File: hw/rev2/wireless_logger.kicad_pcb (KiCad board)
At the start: 4 copper layers, 147 parts, among them J1 FCI 10118194, J2 CONN_2, J3 SSD1306_SER, J4 SWD_10PIN, J5 CONN_5, P1 CONN_6X2, Q1 2N7002P, Q2 2N7002P, U1 MT29FXX01A, U10 CC2541, U11 STM32F40X_BGA176, U2 MAG3110, U3 MMA8452Q, U4 LPS331AP, U5 L3GD20, U6 MCP111T-315, U7 BQ24095, U8 TPS62698, U9 CC1101, X1 FA-128 26.0000MF10Z-W3, X2 9HT10-32.768KBZF-T, X3 FA-128 32.0000MF20X-K3, X4 XRCGB25M000F0L00R0, X5 9HT10-32.768KBZF-T

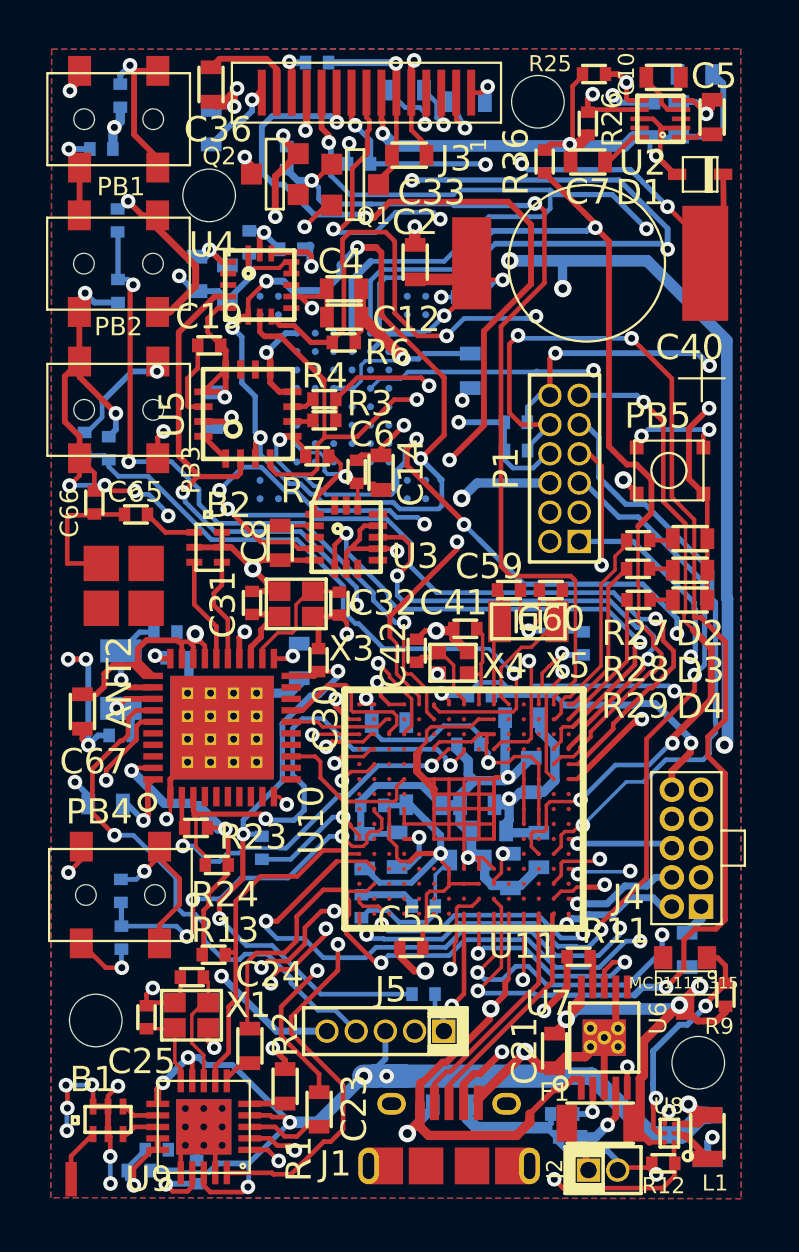
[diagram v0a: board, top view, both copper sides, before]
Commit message: Rev 2a submitted to OSH Park for manufacture
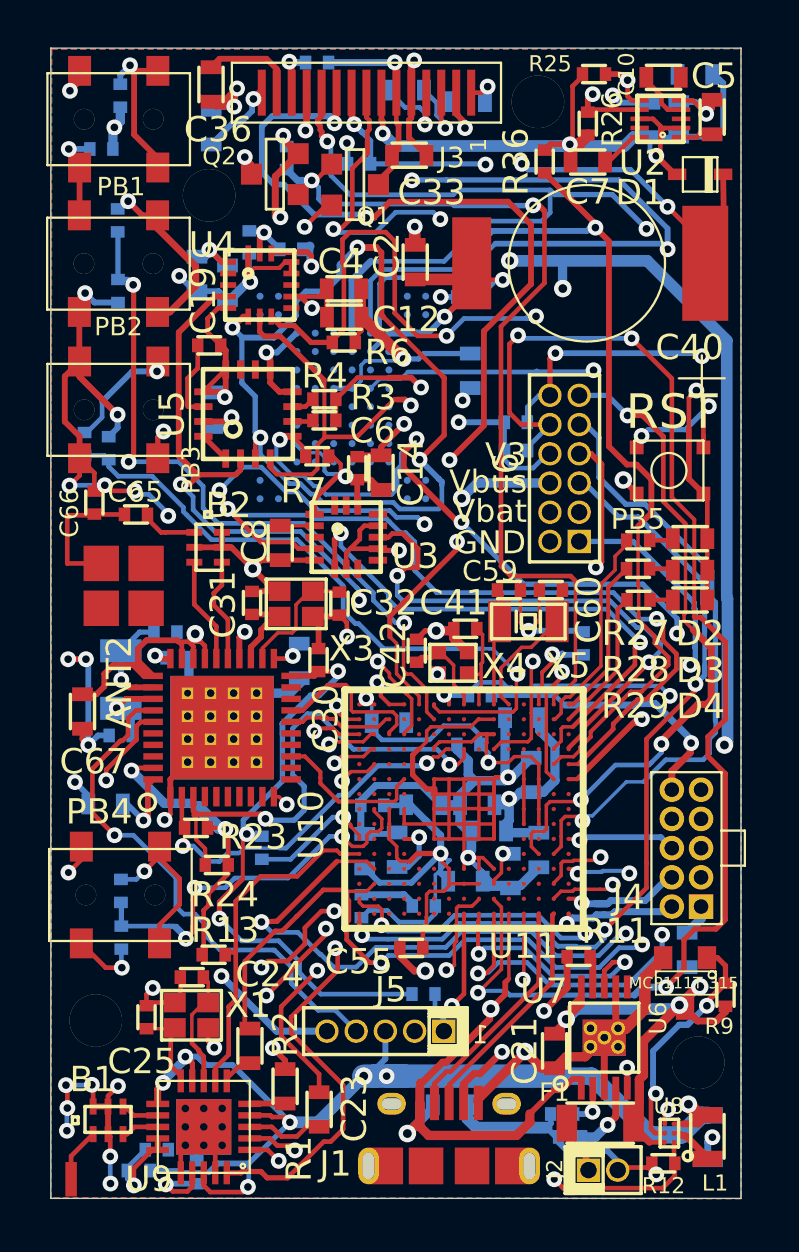
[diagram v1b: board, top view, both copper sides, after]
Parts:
- moved C50 0.92 mm to (188.0, 146.2)
- moved C6 0.16 mm to (183.3, 128.3)
- renumbered P1 to J6
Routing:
- net GND: track 269.3 -> 282.2 mm
- net N-00000167: track 28.6 -> 34.2 mm
- net /Sensors/GYR_SPI_MOSI: track 80.8 -> 85.1 mm, vias 7 -> 6
- net V3: track 328.2 -> 332.4 mm
- net /STM32F4/SPI2_NSS: track 51.5 -> 53.5 mm
- net /STM32F4/EXTI8: track 16.8 -> 18.6 mm
- net N-00000189: track 10.3 -> 12.1 mm
- net /STM32F4/OLED_nD/C: track 47.0 -> 48.6 mm
- net /Sensors/ACC_INT1: track 22.3 -> 23.8 mm
- net /Sensors/ACC_I2C_SCL: track 66.3 -> 67.7 mm
- net /Sensors/GYR_SPI_MISO: track 63.3 -> 62.1 mm
- net /Bluetooth/RF_RESET_N_LOCAL: track 25.8 -> 26.9 mm
- net /OLED/OLED_GND: track 19.3 -> 20.2 mm
- net /OLED/EN: track 39.9 -> 40.8 mm
- net /OLED/SDIN: track 68.1 -> 68.9 mm
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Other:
- board outline added: 30 x 50 mm
- net class 50OHM: via_dia 0.635 -> 0.6858; via_drill 0.3048 -> 0.3302
- net class Default: via_dia 0.635 -> 0.6858; via_drill 0.3048 -> 0.3302
- rule via_min_drill: 0.3048 -> 0.3302
- rule via_min_size: 0.635 -> 0.6858
- board text added: "1"
- board text added: "GND"
- board text added: "RST"
- board text added: "Strike Force rev 2a"
- board text added: "V3"
- board text added: "Vbat"
- board text added: "Vbus"
- board text removed: "rev 2a"
